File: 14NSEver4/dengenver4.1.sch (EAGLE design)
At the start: 46 parts, among them CN1 DM3AT, CN2 DM3AT, Q1 16mhz, Q2 16mhz

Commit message: changed board files
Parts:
- removed BMX1, BMX2: BMX055, BMX055:BMX055
- removed CN1, CN2: DM3AT, microSD:DM3AT
- removed JP2, JP7: (no value), pinhead:PINHD-1X5
- removed L3, L4: (no value), Chip LED:OSXX1608C1A
- removed Q2: 16mhz, crystal:CRYSTALHC49UP
- removed R16, R17, R18, R2, R3, R5, R6: 10k, rcl:R-US_R0603
- removed U$8: ATMEGA328P-AUATMEGA328P-AU, ATMEGA328P-AU:ATMEGA328P-AUATMEGA328P-AU
- added C7: 3.3uF, rcl:C-USC0603
- added CON1, CON3: (no value), XR Connector:3PIN
- added CON2, CON4, CON5: (no value), XR Connector:2PIN
- added D1, D2: (no value), ChipDiodes:1W4148W
- added DCDC1, DCDC3: (no value), DC-DC:5V1A_M78AR05-1
- added DCDC2: (no value), DC-DC:3.3V1A_M78AR033-1
- added IM2: IM920_IM920C, CANSAT12th:IM920_IM920C
- added U$10: 1X61X6_2.5, pin_socket:1X61X6_2.5
- added U$11: 1X5, pin_socket:1X5
- added U$3: 2SK4017-NCH, mosfet:2SK4017-NCH
- C4: value 22p -> 3.3uF
- C5: value 22p -> 10uF
- C6: value 0.1μ -> 3.3uF
- R10, R8: value 10k -> 1k
- R14, R15: value 100 -> 4.7k
- R9: value 10k -> 100k
- SW2: value (none) -> SRIDE_SWITCH; device Tact switch:TVAF06-A020B-R -> Sride Switch:SRIDE_SWITCH
- U$1: value ATMEGA328P-AUATMEGA328P-AU -> 1X5; device ATMEGA328P-AU:ATMEGA328P-AUATMEGA328P-AU -> pin_socket:1X5
- U$2, U$5: value 1X5 -> 2SJ681-PCH; device pin_socket:1X5 -> mosfet:2SJ681-PCH
- U$4: value 1X61X6_2.5 -> 2SJ681-PCH; device pin_socket:1X61X6_2.5 -> mosfet:2SJ681-PCH
- U$7: value 1X61X6_2.5 -> ATMEGA328P-AUATMEGA328P-AU; device pin_socket:1X61X6_2.5 -> ATMEGA328P-AU:ATMEGA328P-AUATMEGA328P-AU
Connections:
- removed net 3V31: BMX2.3V3
- removed net GPSRX: U$1.PD6, U$6.P$4
- removed net GPSTX: U$1.PD7, U$6.P$3
- removed net LED1.0: R15.2, U$1.PD2
- removed net LED1.1: R14.2, U$1.PD3
- removed net LED1.2: R13.2, U$8.PD6
- removed net LED1.3: R12.2, U$8.PD7
- removed net MISO1: CN2.DAT0, R11.1, U$1.PB4, U$7.P$2
- removed net MOSI1: CN2.CMD, R8.1, U$1.PB3, U$7.P$4
- removed net N$11: L3.AN, R14.1
- removed net N$16: C1.1, Q1.1, U$8.PB6
- removed net N$17: C2.1, Q1.2, U$8.PB7
- removed net RESET1: C6.2, U$5.P$3
- removed net RESETB1: C6.1, R16.2, SW2.P$2, U$1.PC6
- removed net RESETTB: U$4.P$5
- removed net RESETTB1: U$7.P$5
- removed net RST: U$1.PD5, U$6.P$5
- removed net RX1: U$1.PD0, U$5.P$4
- removed net SCK1: CN2.CLK, R9.1, U$1.PB5, U$7.P$3
- removed net SCL1: BMX2.SCL, R18.2, U$1.PC5
- removed net SDA1: BMX2.SDA, R17.2, U$1.PC4
- removed net SS1: CN2.CD/DAT3, R5.1
- removed net TX1: U$1.PD1, U$5.P$5
- removed net VCCIO1: BMX2.VCCIO
- new net +5V1: DCDC1.VIN, U$5.DRAIN
- new net FP: CON5.P$1, D2.C, R10.2, U$2.GATE, U$3.GATE, U$4.GATE
- new net FP1: D1.C
- new net FP_CHECKER: C5.1, R8.2, U$7.PD4
- new net IM_BUSY: IM2.BUSY/IO1, U$7.PD6
- new net IM_RESET: IM2.RESET, U$7.PD5
- new net LED: IM2.STATUS
- new net LED_1.0: R13.2, U$7.PD2
- new net LED_1.1: R12.2, U$7.ADC6
- new net N$12: C1.1, Q1.1, U$7.PB6
- new net N$13: C2.1, Q1.2, U$7.PB7
- new net RAW: CON2.P$2, U$2.SOURCE
- new net RX_IM: IM2.RXD/IO6, U$7.PD7
- new net SERVO1: CON1.P$1, R14.1, U$7.PC1
- new net SERVO2: CON3.P$1, R15.1, U$7.PC0
- new net SERVO5V: C7.1, CON1.P$2, CON3.P$2, DCDC3.VOUT
- new net SERVORAW: CON4.P$2, D1.A, DCDC3.VIN
- new net SW: R9.1, SW2.L, U$5.GATE
- new net TX_IM: IM2.TXD/IO7
- new net TX_RM: U$7.PB0
- net +3V3: now also C6.1, DCDC2.VOUT, IM2.VCC, U$1.P$2, U$11.P$1, U$3.DRAIN; no longer CN1.VDD, CN2.VDD, JP2.4, JP7.5, R1.2, R17.1, R18.1, R2.2, R3.2, R5.2, R6.2, R7.2, R8.2, R9.2
- net +5V: now also C4.1, DCDC1.VOUT, DCDC2.VIN, R1.1, R14.2, R15.2, U$1.P$3, U$10.P$1, U$11.P$2, U$7.AVCC, U$7.VCC1, U$7.VCC2; no longer BMX1.VCC, BMX2.VCC, JP2.3, JP7.4, R10.1, R16.1, U$1.AVCC, U$1.VCC1, U$1.VCC2, U$2.P$1, U$4.P$6, U$5.P$1, U$7.P$6, U$8.AVCC, U$8.VCC1, U$8.VCC2
- net BORD1: now also U$1.P$5, U$7.PD3; no longer JP2.1, U$8.PD3
- net BORD2: now also U$1.P$1, U$7.PB1; no longer JP2.5, U$8.PD2
- net BORDRX: now also U$11.P$3, U$7.PC3; no longer JP7.3, U$1.PC3
- net BORDTX: now also U$11.P$4, U$7.PC2; no longer JP7.2, U$1.PC2
- net GND: now also C6.2, C7.2, CON1.P$3, CON2.P$1, CON3.P$3, CON4.P$1, CON5.P$2, DCDC1.GND, DCDC2.GND, DCDC3.GND, IM2.GND, R10.1, R7.1, SW2.LR, U$1.P$4, U$10.P$2, U$11.P$5, U$7.GND1, U$7.GND2, U$7.GND3; no longer BMX1.GND, BMX2.GND, CN1.VSS, CN2.VSS, JP2.2, JP7.1, L3.CT, L4.CT, SW2.P$1, U$1.GND1, U$1.GND2, U$1.GND3, U$2.P$2, U$4.P$1, U$5.P$2, U$7.P$1, U$8.GND1, U$8.GND2, U$8.GND3
- net MISO: now also U$10.P$4, U$7.PB4; no longer CN1.DAT0, R7.1, U$4.P$2, U$8.PB4
- net MOSI: now also U$10.P$5, U$7.PB3; no longer CN1.CMD, R3.1, U$4.P$4, U$8.PB3
- net N$14: now also R7.2, R8.1, U$3.SOURCE; no longer C5.1, Q2.2, U$1.PB7
- net N$2: now also U$2.DRAIN, U$4.DRAIN; no longer L4.AN, R15.1
- net N$3: now also D2.A, R9.2, U$4.SOURCE, U$5.SOURCE; no longer C4.1, Q2.1, U$1.PB6
- net RESET: now also U$6.P$3; no longer U$2.P$3
- net RESETB: now also R1.2, U$10.P$6, U$7.PC6; no longer R10.2, U$8.PC6
- net RX: now also U$6.P$4, U$7.PD0; no longer U$2.P$4, U$8.PD0
- net SCK: now also U$10.P$3, U$7.PB5; no longer CN1.CLK, R6.1, U$4.P$3, U$8.PB5
- net SCL: now also R11.1, U$7.PC5; no longer BMX1.SCL, R4.1, U$8.PC5
- net SDA: now also R4.1, U$7.PC4; no longer BMX1.SDA, R2.1, U$8.PC4
- net SS: now also U$7.PB2; no longer CN1.CD/DAT3, R1.1, U$1.PB2, U$8.PB2
- net TX: now also U$6.P$5, U$7.PD1; no longer U$2.P$5, U$8.PD1
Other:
- note added: "PWR"
- moved on the sheet: BMP1, C1, C2, C3, C4, C5, C6, L1, L2, Q1, R1, R10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

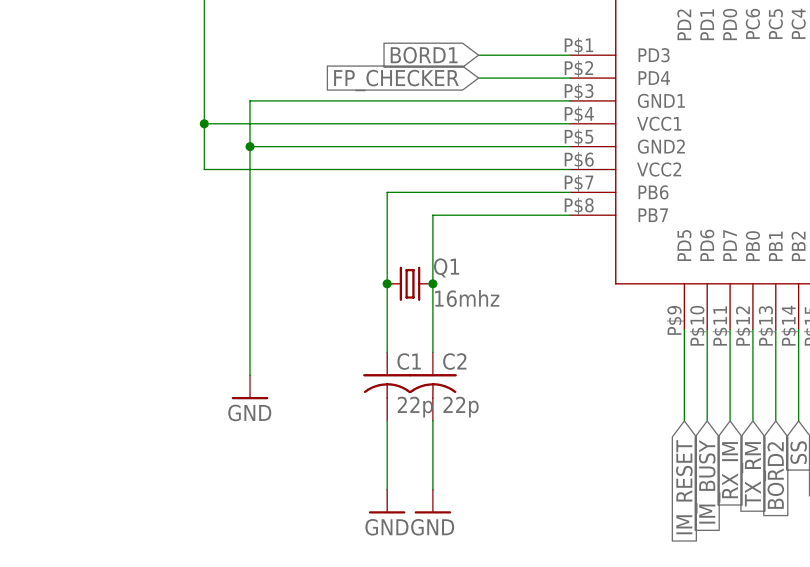
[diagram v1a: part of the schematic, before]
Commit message: changed v4.2
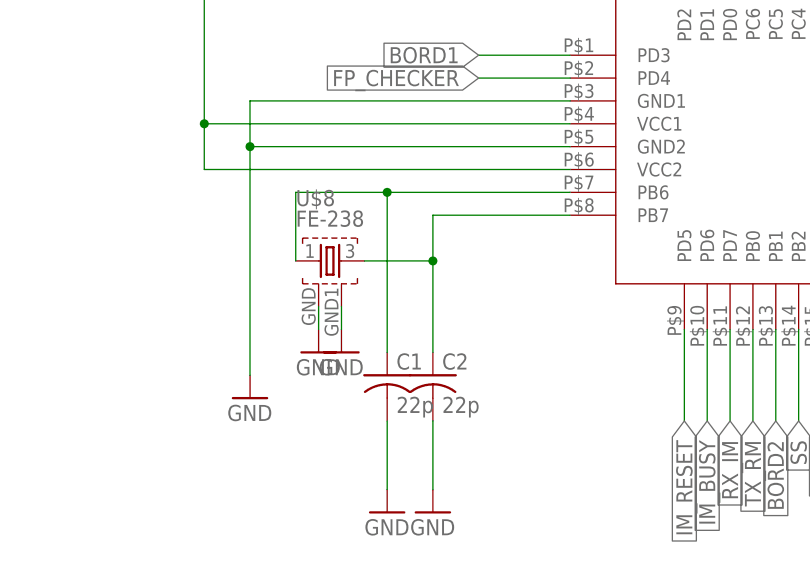
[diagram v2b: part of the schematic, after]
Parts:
- removed Q1: 16mhz, crystal:CRYSTALHC49UP
- added U$8: FE-238, FA-238:FE-238
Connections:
- net GND: now also U$8.GND, U$8.GND1
- net N$12: now also U$8.1; no longer Q1.1
- net N$13: now also U$8.3; no longer Q1.2
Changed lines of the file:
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@@
 <parts>
 <part name="R1" library="rcl" library_urn="urn:adsk.eagle:library:334" deviceset="R-US_" device="R0603" package3d_urn="urn:adsk.eagle:package:23555/3" value="10k"/>
-<part name="Q1" library="crystal" library_urn="urn:adsk.eagle:library:204" deviceset="CRYSTAL" device="HC49UP" package3d_urn="urn:adsk.eagle:package:12078/1" value="16mhz"/>
 <part name="C1" library="rcl" library_urn="urn:adsk.eagle:library:334" deviceset="C-US" device="C1608" package3d_urn="urn:adsk.eagle:package:23621/2" value="22p"/>
 <part name="C2" library="rcl" library_urn="urn:adsk.eagle:library:334" deviceset="C-US" device="C1608" package3d_urn="urn:adsk.eagle:package:23621/2" value="22p"/>
@@
 <part name="U$6" library="pin_socket" deviceset="1X5" device="" package3d_urn="urn:adsk.eagle:package:44791100/1"/>
 <part name="U$7" library="ATMEGA328P-AU" deviceset="ATMEGA328P-AU" device="ATMEGA328P-AU"/>
+<part name="U$8" library="FA-238" library_urn="urn:adsk.eagle:library:44894307" deviceset="FE-238" device="" package3d_urn="urn:adsk.eagle:package:44894250/2"/>
+<part name="GND3" library="supply1" library_urn="urn:adsk.eagle:library:371" deviceset="GND" device=""/>
+<part name="GND7" library="supply1" library_urn="urn:adsk.eagle:library:371" deviceset="GND" device=""/>
 </parts>
 <sheets>
@@
 <attribute name="VALUE" x="143.51" y="77.978" size="1.778" layer="96"/>
 </instance>
-<instance part="Q1" gate="G$1" x="147.32" y="20.32" smashed="yes">
-<attribute name="NAME" x="149.86" y="21.336" size="1.778" layer="95"/>
-<attribute name="VALUE" x="149.86" y="17.78" size="1.778" layer="96"/>
-</instance>
 <instance part="C1" gate="G$1" x="144.78" y="10.16" smashed="yes">
 <attribute name="NAME" x="145.796" y="10.795" size="1.778" layer="95"/>
@@
 </instance>
 <instance part="U$7" gate="G$1" x="170.18" y="53.34" smashed="yes"/>
+<instance part="U$8" gate="G$1" x="137.16" y="22.86" smashed="yes">
+<attribute name="NAME" x="134.62" y="28.956" size="1.778" layer="95"/>
+<attribute name="VALUE" x="134.62" y="26.67" size="1.778" layer="96"/>
+</instance>
+<instance part="GND3" gate="1" x="137.16" y="12.7" smashed="yes">
+<attribute name="VALUE" x="134.62" y="10.16" size="1.778" layer="96"/>
+</instance>
+<instance part="GND7" gate="1" x="139.7" y="12.7" smashed="yes">
+<attribute name="VALUE" x="137.16" y="10.16" size="1.778" layer="96"/>
+</instance>
 </instances>
 <busses>
@@
 <pinref part="GND23" gate="1" pin="GND"/>
 <pinref part="U$7" gate="G$1" pin="GND3"/>
+</segment>
+<segment>
+<pinref part="U$8" gate="G$1" pin="GND"/>
+<wire x1="137.16" y1="15.24" x2="137.16" y2="17.78" width="0.1524" layer="91"/>
+<pinref part="GND3" gate="1" pin="GND"/>
+</segment>
+<segment>
+<pinref part="U$8" gate="G$1" pin="GND1"/>
+<wire x1="139.7" y1="15.24" x2="139.7" y2="17.78" width="0.1524" layer="91"/>
+<pinref part="GND7" gate="1" pin="GND"/>
 </segment>
 </net>
@@
 <net name="N$12" class="0">
 <segment>
-<pinref part="Q1" gate="G$1" pin="1"/>
-<wire x1="144.78" y1="20.32" x2="144.78" y2="12.7" width="0.1524" layer="91"/>
-<junction x="144.78" y="20.32"/>
 <pinref part="C1" gate="G$1" pin="1"/>
-<wire x1="144.78" y1="20.32" x2="144.78" y2="30.48" width="0.1524" layer="91"/>
+<wire x1="144.78" y1="12.7" x2="144.78" y2="30.48" width="0.1524" layer="91"/>
 <wire x1="144.78" y1="30.48" x2="165.1" y2="30.48" width="0.1524" layer="91"/>
 <pinref part="U$7" gate="G$1" pin="PB6"/>
+<pinref part="U$8" gate="G$1" pin="1"/>
+<wire x1="134.62" y1="22.86" x2="134.62" y2="30.48" width="0.1524" layer="91"/>
+<wire x1="134.62" y1="30.48" x2="144.78" y2="30.48" width="0.1524" layer="91"/>
+<junction x="144.78" y="30.48"/>
 </segment>
 </net>
 <net name="N$13" class="0">
 <segment>
-<pinref part="Q1" gate="G$1" pin="2"/>
-<wire x1="149.86" y1="20.32" x2="149.86" y2="12.7" width="0.1524" layer="91"/>
-<junction x="149.86" y="20.32"/>
+<wire x1="149.86" y1="22.86" x2="149.86" y2="12.7" width="0.1524" layer="91"/>
 <pinref part="C2" gate="G$1" pin="1"/>
 <wire x1="165.1" y1="27.94" x2="149.86" y2="27.94" width="0.1524" layer="91"/>
-<wire x1="149.86" y1="20.32" x2="149.86" y2="27.94" width="0.1524" layer="91"/>
 <pinref part="U$7" gate="G$1" pin="PB7"/>
+<pinref part="U$8" gate="G$1" pin="3"/>
+<wire x1="149.86" y1="22.86" x2="149.86" y2="27.94" width="0.1524" layer="91"/>
+<wire x1="142.24" y1="22.86" x2="149.86" y2="22.86" width="0.1524" layer="91"/>
+<junction x="149.86" y="22.86"/>
 </segment>
 </net>
